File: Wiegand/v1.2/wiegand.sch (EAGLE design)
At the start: 58 parts, among them CON1 SPI, Q1 BCP69, Q2 BCP69, Q3 BCP69, Q4 BCP69, Q5 BCP69, X3 16MHz, X4 MINI-USB

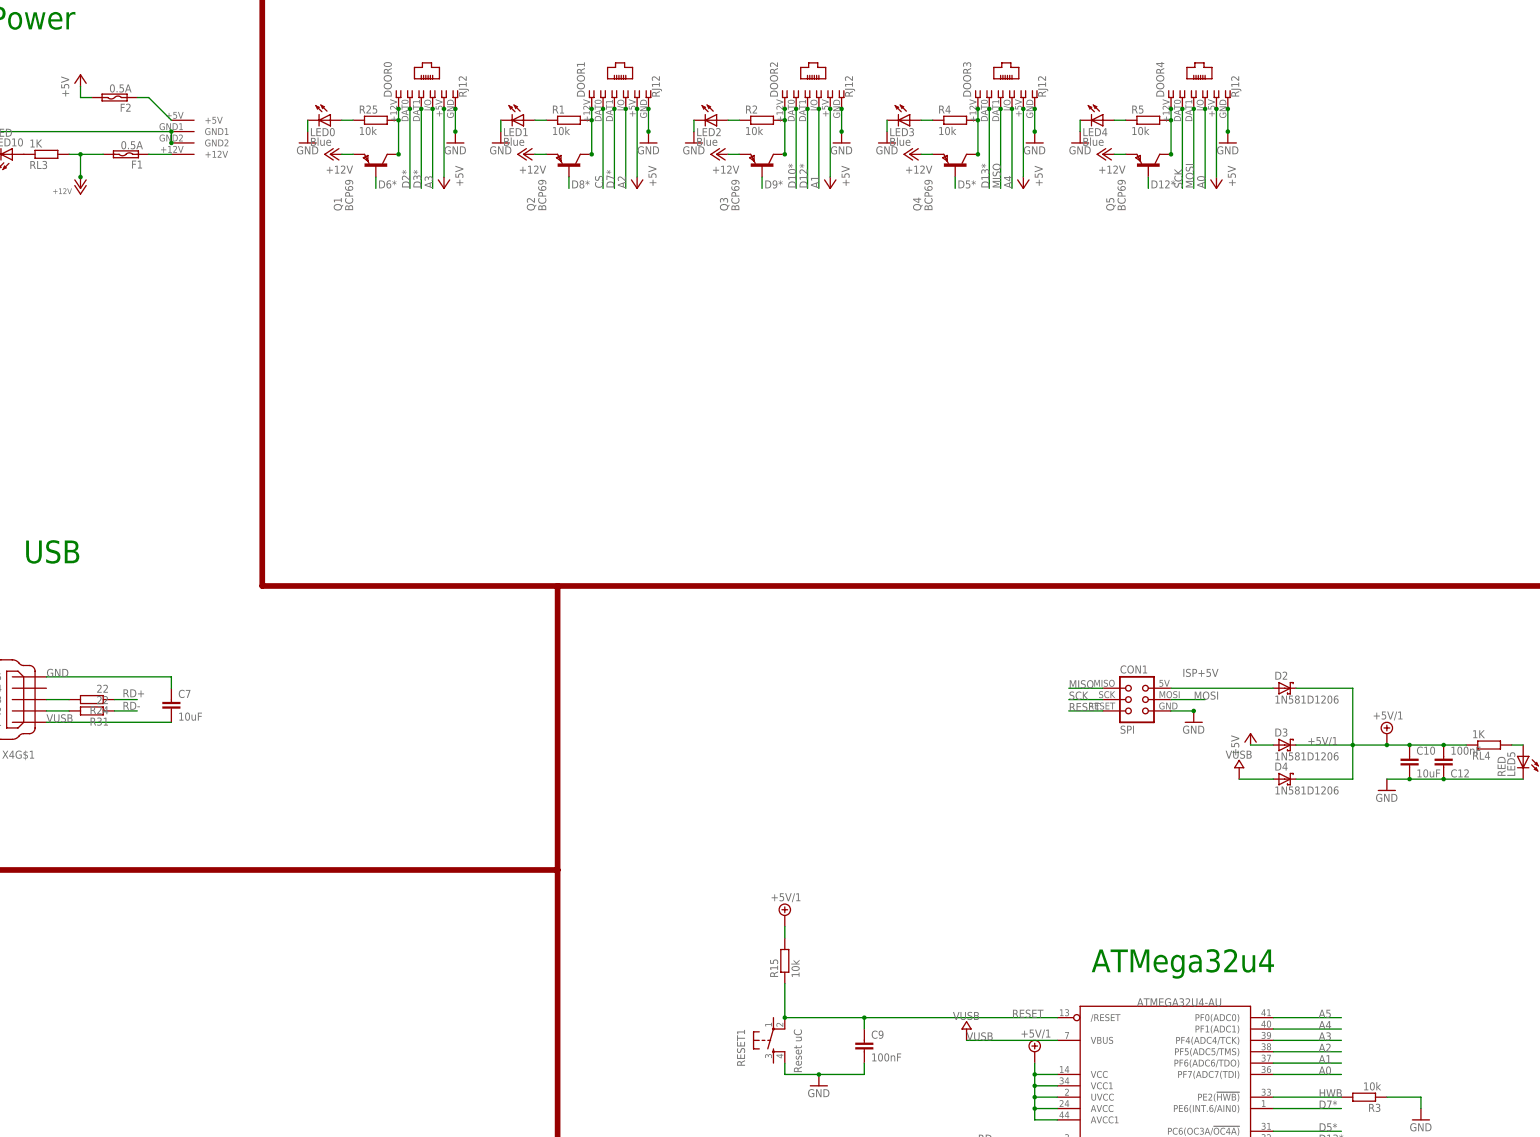
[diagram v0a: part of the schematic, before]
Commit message: New version based on BSP 75
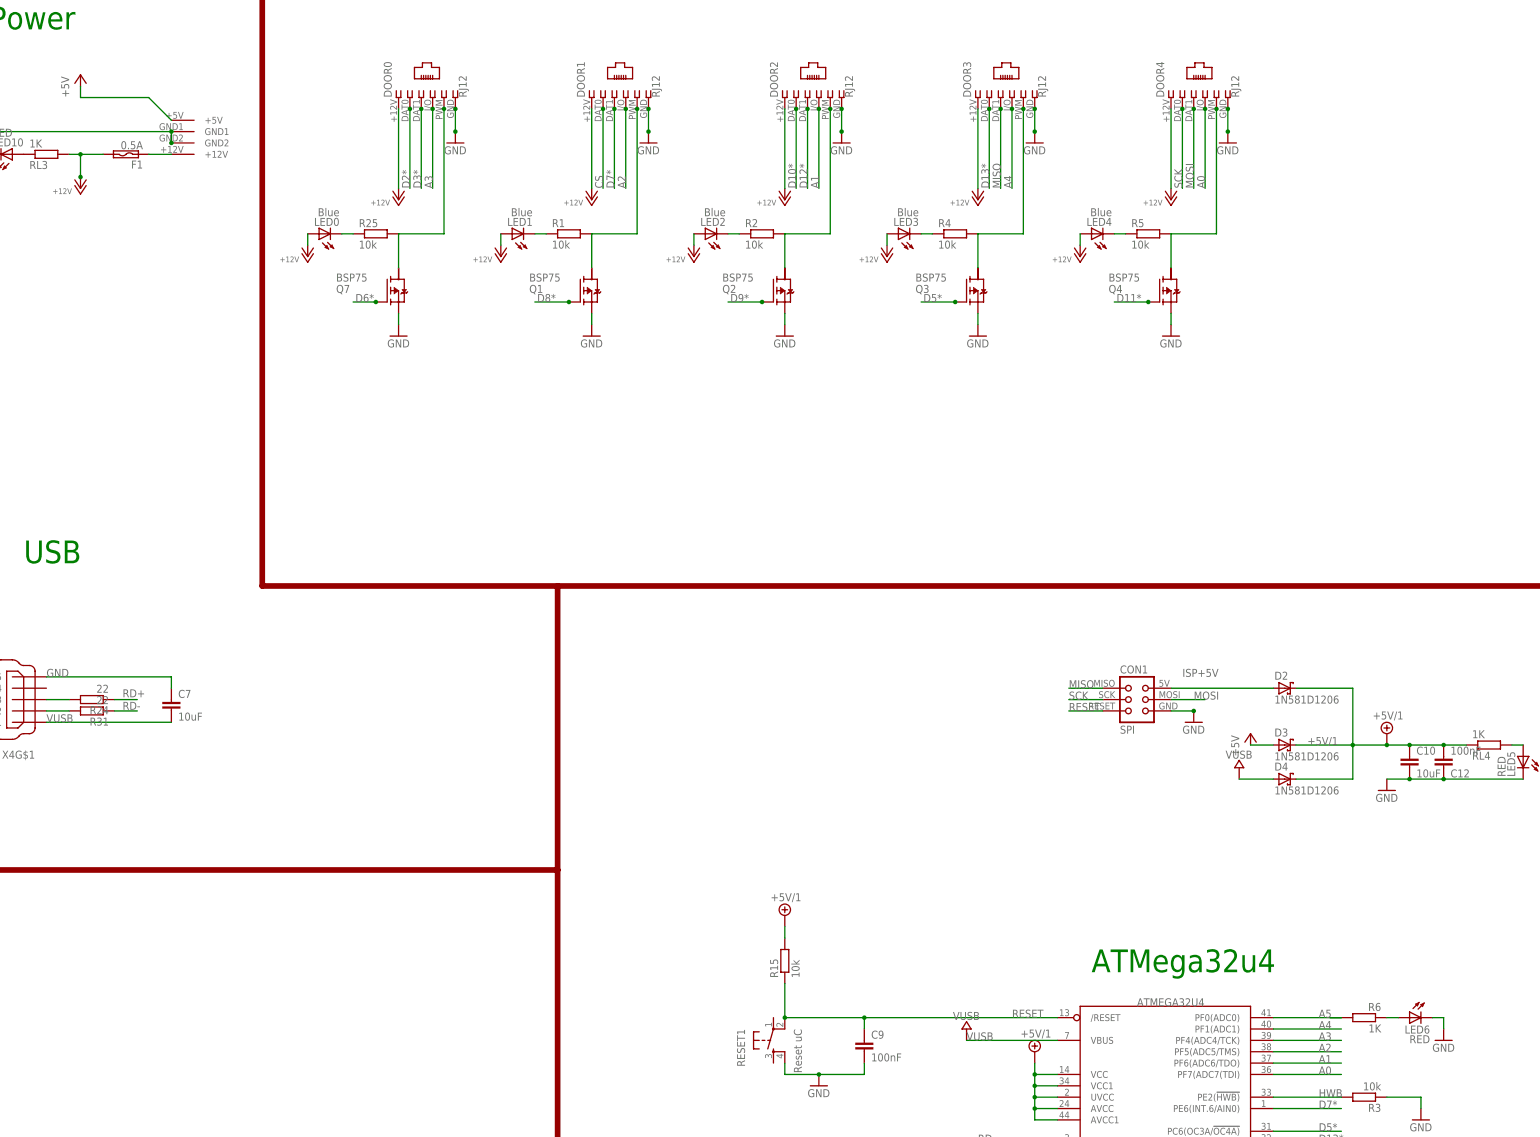
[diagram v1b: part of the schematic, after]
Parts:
- removed F2: 0.5A, lpatiny:POLYSWITCHSMD1812
- removed Q5: BCP69, zetex:PNPSOT223
- added LED6: RED, SparkFun:LED1206
- added Q7: BSP75, infineon:BSP613P
- added R6: 1K, rcl:R-EU_R0805
- Q1, Q2, Q3, Q4: value BCP69 -> BSP75; device zetex:PNPSOT223 -> infineon:BSP613P
- U$4: value ATMEGA32U4-AU -> ATMEGA32U4
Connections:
- removed net N$17: LED0.A, R25.1
- removed net N$19: LED3.A, R4.1
- removed net N$29: LED4.A, R5.1
- removed net N$38: F2.1, U$6.+5V
- new net +5V1: R6.2
- new net N$2: LED6.A, R6.1
- new net N$6: LED2.C, R2.1
- new net N$8: LED3.C, R4.1
- new net N$9: LED4.C, R5.1
- net +12V: now also DOOR0.1, DOOR1.1, DOOR2.1, DOOR3.1, DOOR4.1, LED0.A, LED1.A, LED2.A, LED3.A, LED4.A; no longer Q1.E, Q2.E, Q3.E, Q4.E, Q5.E
- net +5V: now also U$6.+5V; no longer DOOR0.5, DOOR1.5, DOOR2.5, DOOR3.5, DOOR4.5, F2.2
- net D11*: now also Q4.G
- net D12*: no longer Q5.B
- net D5*: now also Q3.G; no longer Q4.B
- net D6*: now also Q7.G; no longer Q1.B
- net D8*: now also Q1.G; no longer Q2.B
- net D9*: now also Q2.G; no longer Q3.B
- net GND: now also LED6.C, Q1.S, Q2.S, Q3.S, Q4.S, Q7.S; no longer LED0.C, LED1.C, LED2.C, LED3.C, LED4.C
- net N$1: now also LED0.C, R25.1; no longer LED1.A, R1.1
- net N$22: now also DOOR3.5, Q3.D@1; no longer DOOR3.1, Q4.C
- net N$23: now also DOOR0.5, Q7.D@1; no longer DOOR0.1, Q1.C
- net N$3: now also DOOR1.5, Q1.D@1; no longer DOOR1.1, Q2.C
- net N$31: now also DOOR4.5, Q4.D@1; no longer DOOR4.1, Q5.C
- net N$5: now also LED1.C, R1.1; no longer LED2.A, R2.1
- net N$7: now also DOOR2.5, Q2.D@1; no longer DOOR2.1, Q3.C
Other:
- moved on the sheet: LED0, LED1, LED2, LED3, LED4, R1, R2, R25, R4, R5
